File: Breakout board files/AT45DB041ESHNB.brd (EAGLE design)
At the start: 22.7 x 17.7 mm, 9 parts, among them U1 AT45DB041E-SHN-B

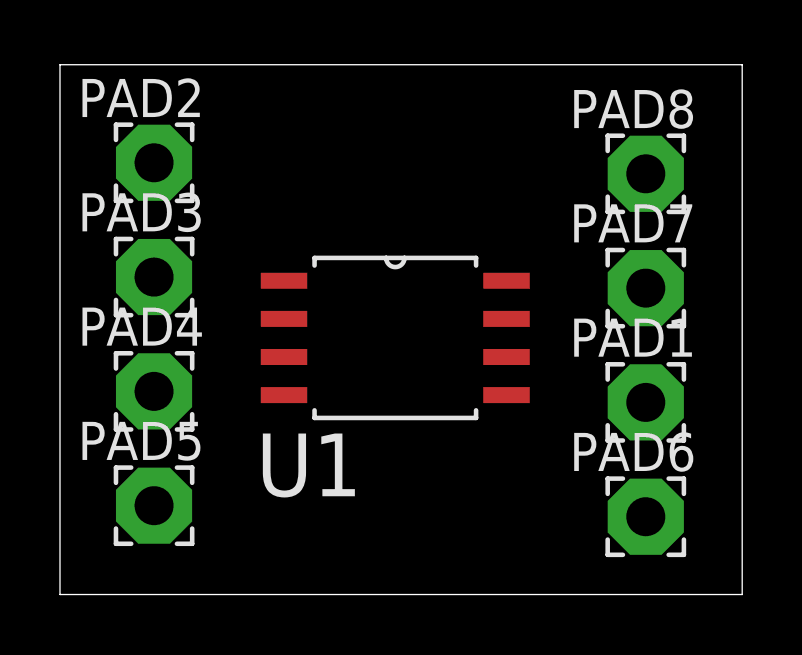
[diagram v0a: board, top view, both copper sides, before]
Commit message: Breakout Board Solutions
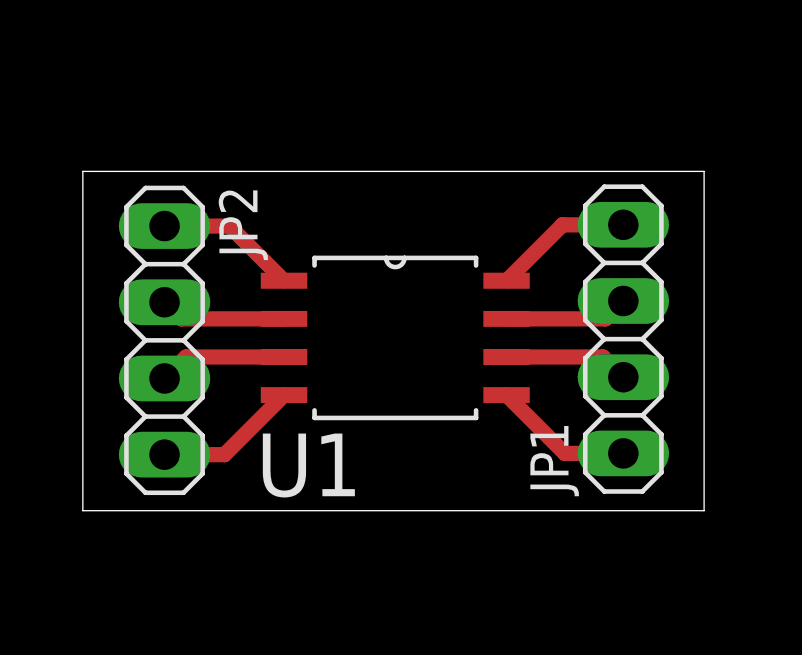
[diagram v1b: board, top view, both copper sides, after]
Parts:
- removed PAD1, PAD2, PAD3, PAD4, PAD5, PAD6, PAD7, PAD8: (no value), ee2parts:2,54/1,1
- added JP1, JP2: (no value), pinhead:1X04
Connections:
- removed net N$1: PAD1.1, U1.6
- removed net N$2: PAD2.1, U1.1
- removed net N$3: PAD3.1, U1.2
- removed net N$4: PAD4.1, U1.3
- removed net N$5: PAD5.1, U1.4
- removed net N$6: PAD6.1, U1.5
- removed net N$7: PAD7.1, U1.7
- removed net N$8: PAD8.1, U1.8
- new net 1: JP2.1, U1.1
- new net 2: JP2.2, U1.2
- new net 3: JP2.3, U1.3
- new net 4: JP2.4, U1.4
- new net 5: JP1.1, U1.5
- new net 6: JP1.2, U1.6
- new net 7: JP1.3, U1.7
- new net 8: JP1.4, U1.8
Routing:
- net 4: track 0.00 -> 4.81 mm
- net 1: track 0.00 -> 4.74 mm
- net 5: track 0.00 -> 4.70 mm
- net 8: track 0.00 -> 4.67 mm
- net 3: track 0.00 -> 4.28 mm
- net 2: track 0.00 -> 4.21 mm
- net 6: track 0.00 -> 4.17 mm
- net 7: track 0.00 -> 4.14 mm
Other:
- board size 22.7 x 17.7 mm -> 20.7 x 11.3 mm
